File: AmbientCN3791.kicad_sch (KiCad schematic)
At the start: 55 parts, among them J1 Conn_01x02, J2 Conn_01x02, J3 Conn_01x02, J4 Conn_01x04, J5 Conn_01x04, J6 Conn_01x02, Q1 AO4813, SW1 SW_SPDT, U1 CN3791, U2 INA3221

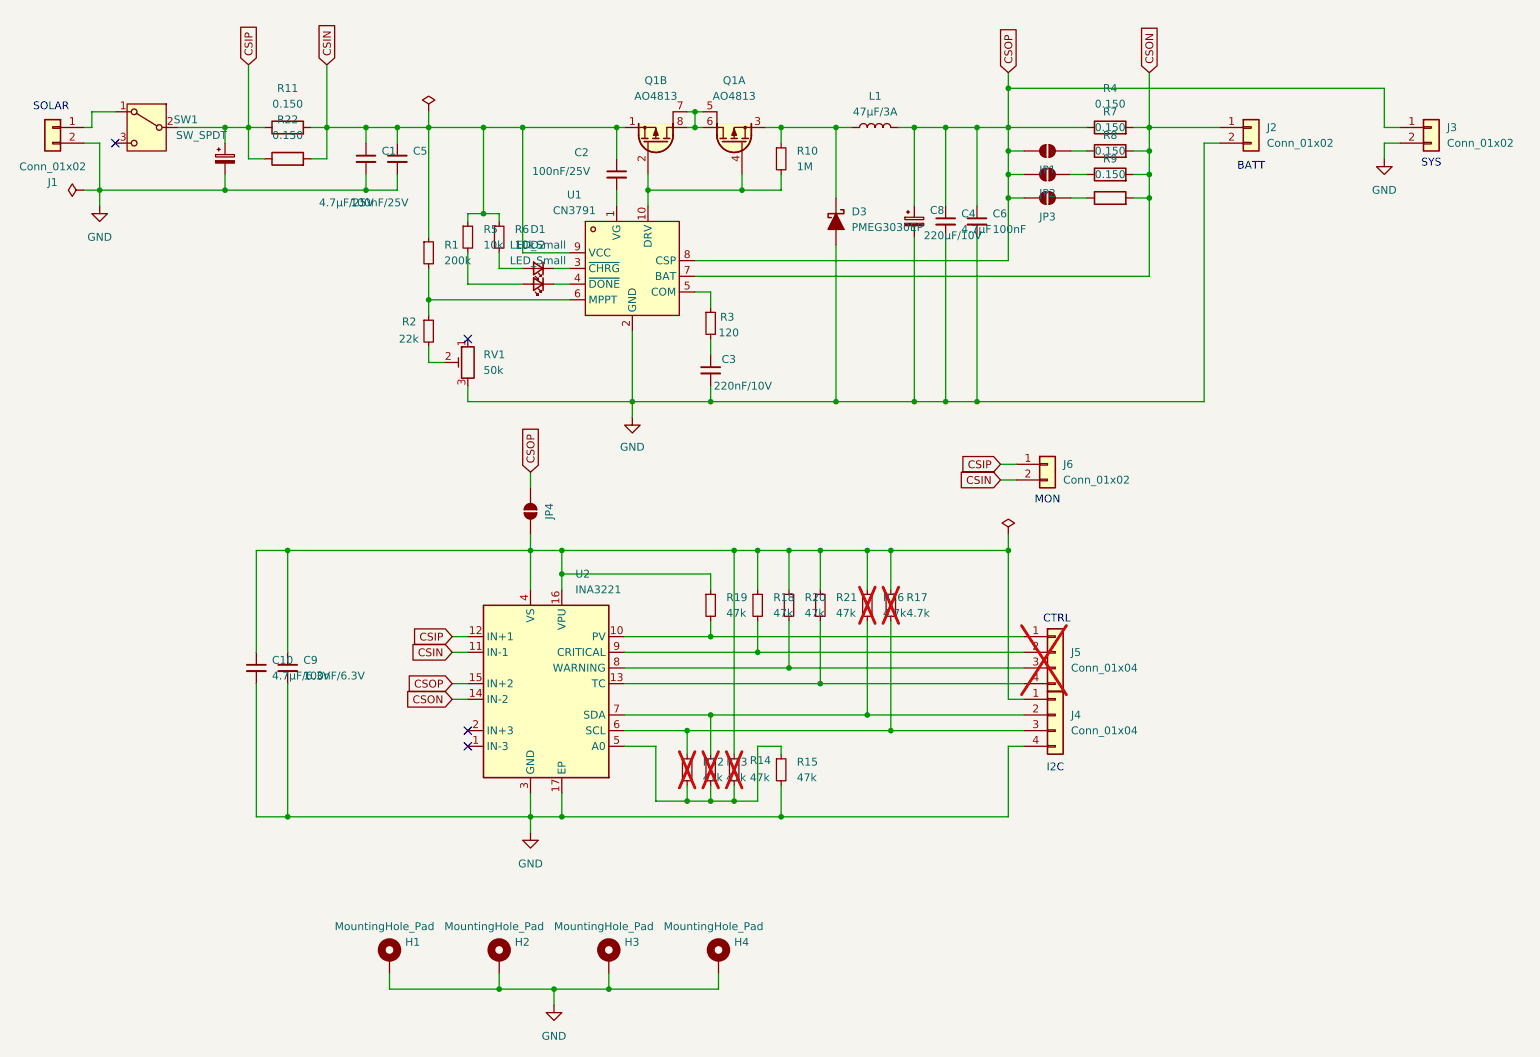
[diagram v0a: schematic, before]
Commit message: AmbientCN3791 v0.1
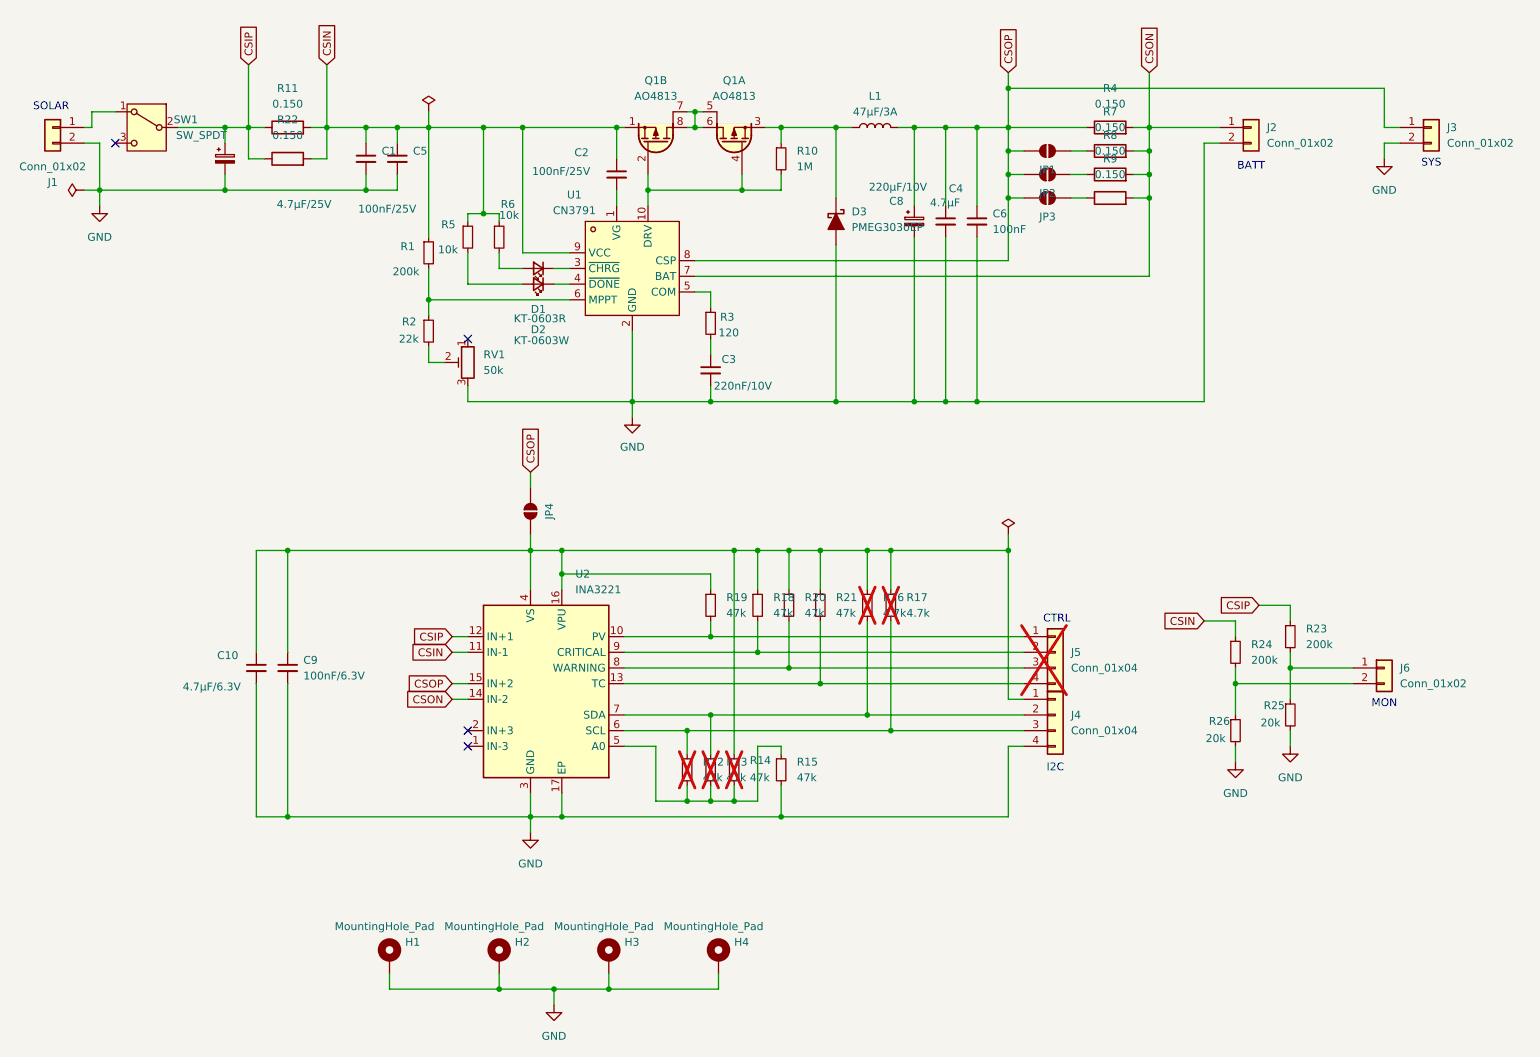
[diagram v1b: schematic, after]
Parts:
- added R23, R24: 200k, Resistor_SMD:R_0402_1005Metric, symbol Device:R_Small
- added R25, R26: 20k, Resistor_SMD:R_0402_1005Metric, symbol Device:R_Small
- C1, C10, C4: LCSC (none) -> C1779
- C2, C5, C6, C9: LCSC (none) -> C307331
- C3: LCSC (none) -> C16772
- C7, C8: JLCPCB Rotation Offset (none) -> 180
- D1: value LED_Small -> KT-0603R
- D2: value LED_Small -> KT-0603W; LCSC (none) -> C2290
- J1, J2, J3, J6: JLCPCB Position Offset (none) -> 0,3.6195; JLCPCB Rotation Offset (none) -> 180; LCSC (none) -> C157931
- J4: JLCPCB Position Offset (none) -> 0,-3.429; LCSC (none) -> C157925
- Q1, RV1: JLCPCB Rotation Offset (none) -> -90
- R10: LCSC (none) -> C26083
- R2: LCSC (none) -> C25768
- R3: LCSC (none) -> C25079
- R5: LCSC C2297 -> C25744
- R6: LCSC (none) -> C25744
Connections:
- net CSIN: now also R24.1; no longer J6.2 (Pin_2)
- net CSIP: now also R23.1; no longer J6.1 (Pin_1)
- net GND: now also R25.2, R26.2
- new net: J6.2 (Pin_2), R24.2, R26.1
- new net: J6.1 (Pin_1), R23.2, R25.1
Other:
- moved on the sheet: J6
